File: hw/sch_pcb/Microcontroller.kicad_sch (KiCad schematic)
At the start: 28 parts, among them J1 HEADER_2x01_PARALLEL, J2 HEADER_2x01, J3 HEADER_2x03, U1 ISL21080CIH320Z-TK, U2 LM4041CIM3-1.2(neosazovat), U3 ATMEGA1284P-AU, Y6 8MHz LFXTAL083138

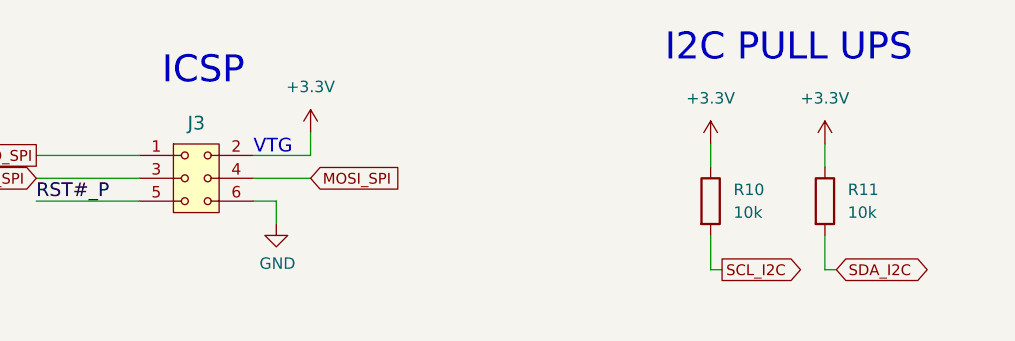
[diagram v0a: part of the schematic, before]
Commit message: Desing improvements WIP.
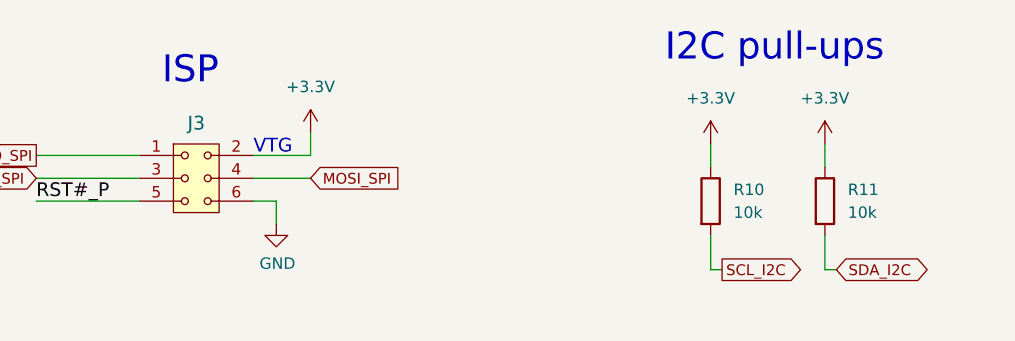
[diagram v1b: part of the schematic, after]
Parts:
- J3: footprint Mlab_Pin_Headers:Straight_2x03 -> Mlab_Pin_Headers:SMD_2x03_WO_paste
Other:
- note added: "I2C pull-ups"
- note added: "ISP"
- note removed: "I2C PULL UPS"
- note removed: "ICSP"
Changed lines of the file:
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@@
 		)
 	)
-	(text "I2C PULL UPS"
+	(text "I2C pull-ups"
 		(exclude_from_sim no)
 		(at 233.68 21.59 0)
@@
 		)
 	)
-	(text "ICSP"
+	(text "ISP"
 		(exclude_from_sim no)
 		(at 177.8 24.13 0)
@@
 			)
 		)
-		(property "Footprint" "Mlab_Pin_Headers:Straight_2x03"
+		(property "Footprint" "Mlab_Pin_Headers:SMD_2x03_WO_paste"
 			(at 181.61 31.75 0)
 			(effects
@@
 			(at 181.61 34.29 0)
 			(effects
+				(font
+					(size 1.27 1.27)
+				)
+				(hide yes)
+			)
+		)
+		(property "UST_ID" ""
+			(at 181.61 34.29 0)
+			(effects
